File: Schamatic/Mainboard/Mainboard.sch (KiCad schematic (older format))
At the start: 104 parts, among them J1 BAT+, J10 BAT-, J11 PLUG+, J12 PLUG-, J13 MOUNT, J14 MOUNT, J15 MOUNT, J16 MOUNT, J2 M+1, J3 USART, J4 3.3V, J5 CONN_02X04, J6 JTAG, J7 M+2, J8 M-1, J9 M-2, Q1 p-MOSFET, SW1 B3U-1000P, SW2 B3U-1000P, SW3 B3U-1000P, SW4 B3U-1000P, SW5 B3U-1000P, U1 ACS781, U2 ADP2303ARDZ-3.3, U3 cc3220, U4 DEA202450BT-3201B2, U5 MX25R3235F, U6 LSM9DS1, U7 LTC2954, U8 LTC2876, Y1 32.768kHz, Y2 40Mhz

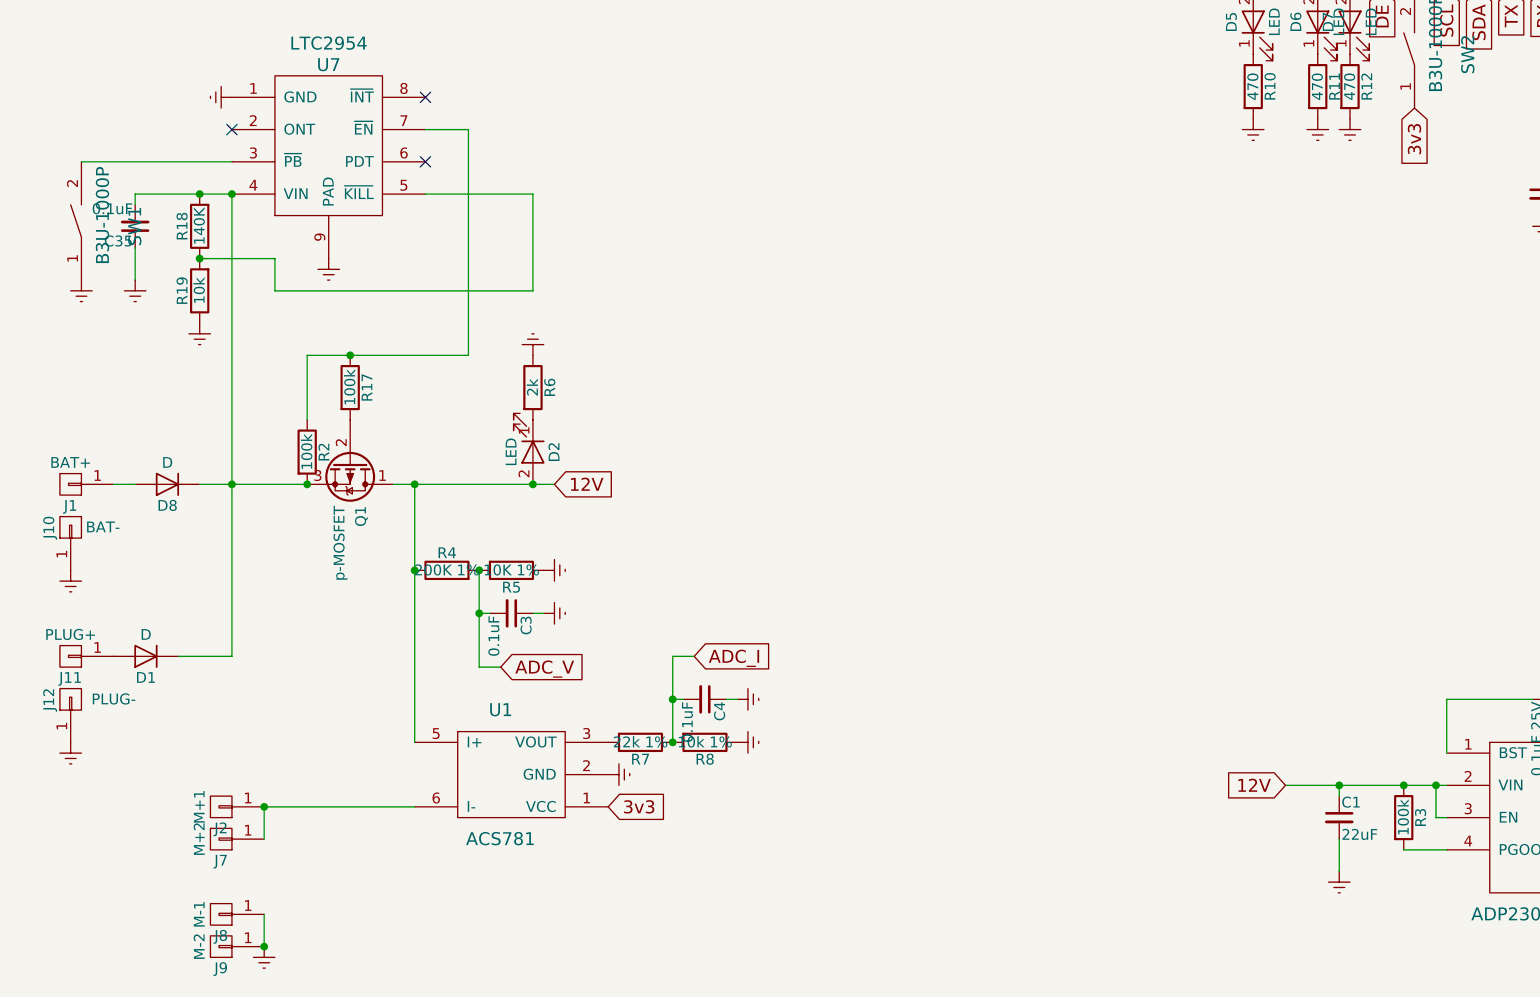
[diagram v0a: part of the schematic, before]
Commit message: BAU
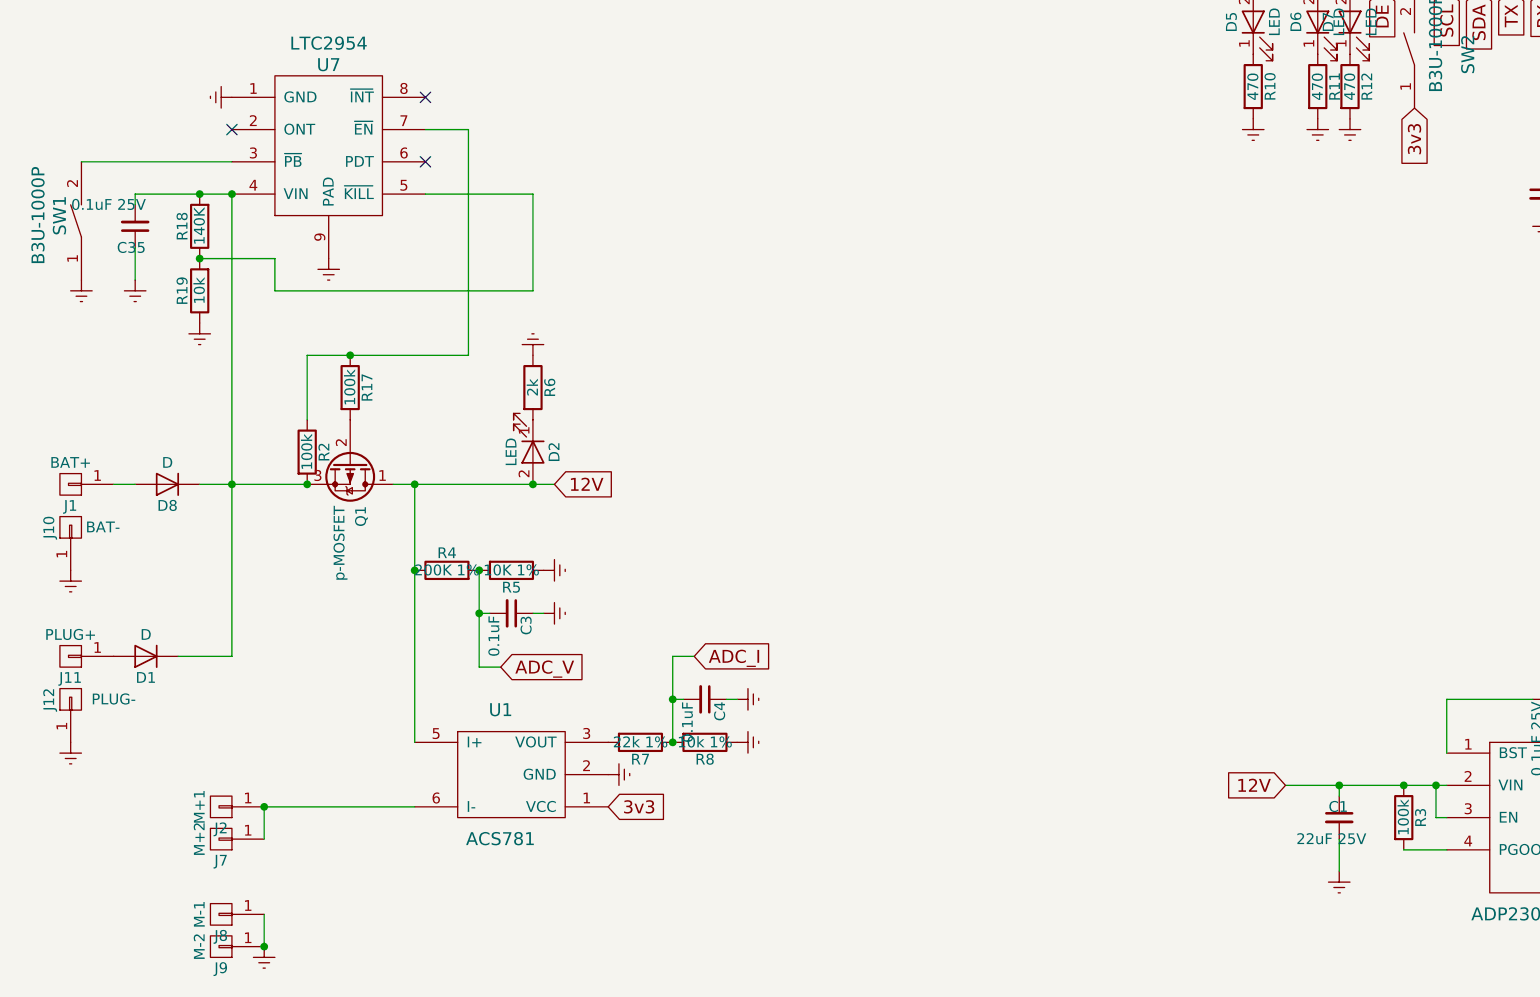
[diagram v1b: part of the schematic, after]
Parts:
- C1: value 22uF -> 22uF 25V
- C35: value 0.1uF -> 0.1uF 25V
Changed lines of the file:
@@
 U 1 1 5A43873A
 P 6750 10050
-F 0 "C1" H 6760 10120 50  0000 L CNN
-F 1 "22uF" H 6760 9970 50  0000 L CNN
+F 0 "C1" H 6700 10100 50  0000 L CNN
+F 1 "22uF 25V" H 6550 9950 50  0000 L CNN
 F 2 "Capacitors_SMD:C_0805" H 6750 10050 50  0001 C CNN
 F 3 "" H 6750 10050 50  0001 C CNN
@@
 U 1 1 5A43A034
 P 1450 7250
-F 0 "SW1" H 1400 7550 60  0000 C CNN
-F 1 "B3U-1000P" H 1450 7700 60  0000 C CNN
+F 0 "SW1" H 1450 7900 60  0000 C CNN
+F 1 "B3U-1000P" H 1450 8000 60  0000 C CNN
 F 2 "Resistors_SMD:R_1206" H 1450 7250 60  0001 C CNN
 F 3 "" H 1450 7250 60  0001 C CNN
@@
 U 1 1 5A4BBA39
 P 1150 7300
-F 0 "C35" H 1160 7370 50  0000 L CNN
-F 1 "0.1uF" H 1160 7220 50  0000 L CNN
+F 0 "C35" H 1100 7400 50  0000 L CNN
+F 1 "0.1uF 25V" H 1100 7200 50  0000 L CNN
 F 2 "Capacitors_SMD:C_0603" H 1150 7300 50  0001 C CNN
 F 3 "" H 1150 7300 50  0001 C CNN
